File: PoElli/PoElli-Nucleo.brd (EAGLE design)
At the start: 79.5 x 70 mm, 122 parts, among them CN10 NUCLEO-CN10, CN7 NUCLEO-CN7, J3 M022.54MM, J4 M022.54MM, Q3 FDMC2674, Q4 IRFL4310, SW1 A6H2101, SW2 A6H2101, T1 Coilcraft 230NL, T2 FLYBACK750311689, U4 LT3748, U5 TPS2378, U6 ENC424J600, X1 POE-TP-SHIELDED-RJ45-MOLEX-85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, Y1 25 MHz

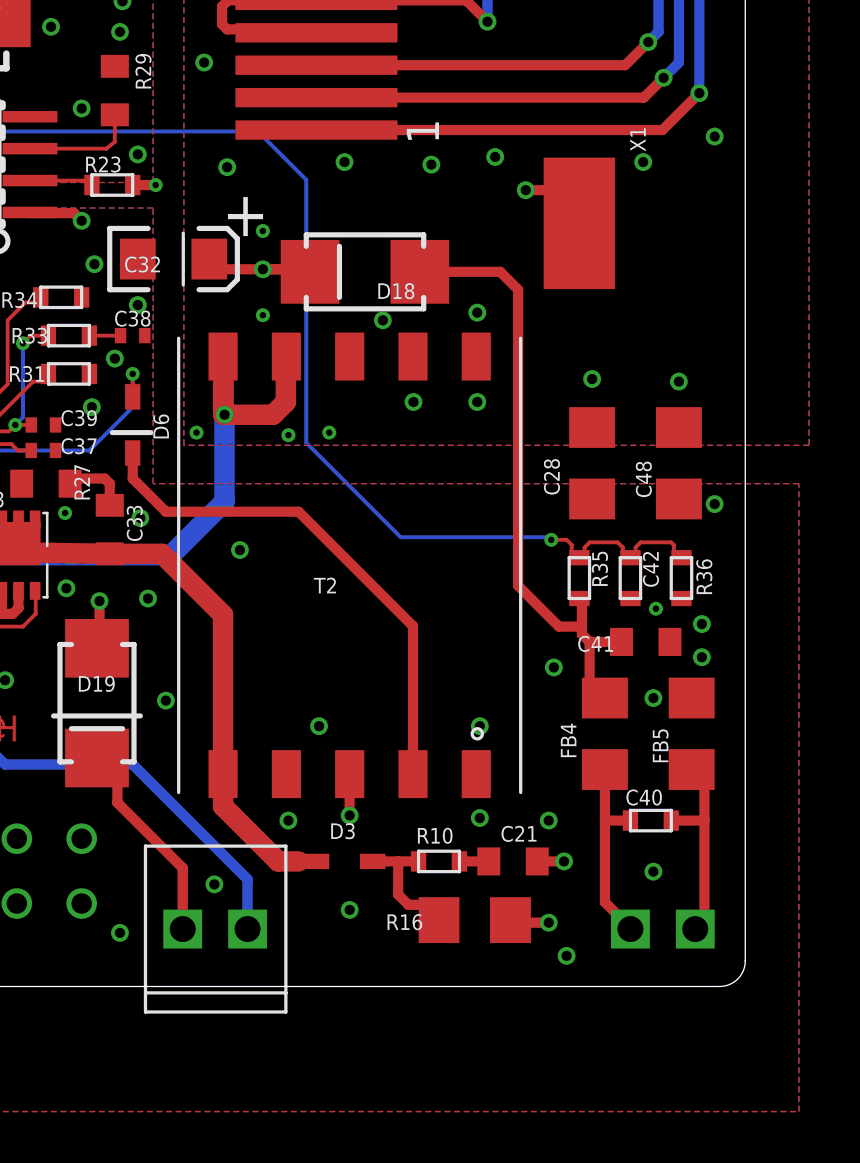
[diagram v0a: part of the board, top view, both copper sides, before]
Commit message: final tweakings, draft v0.9
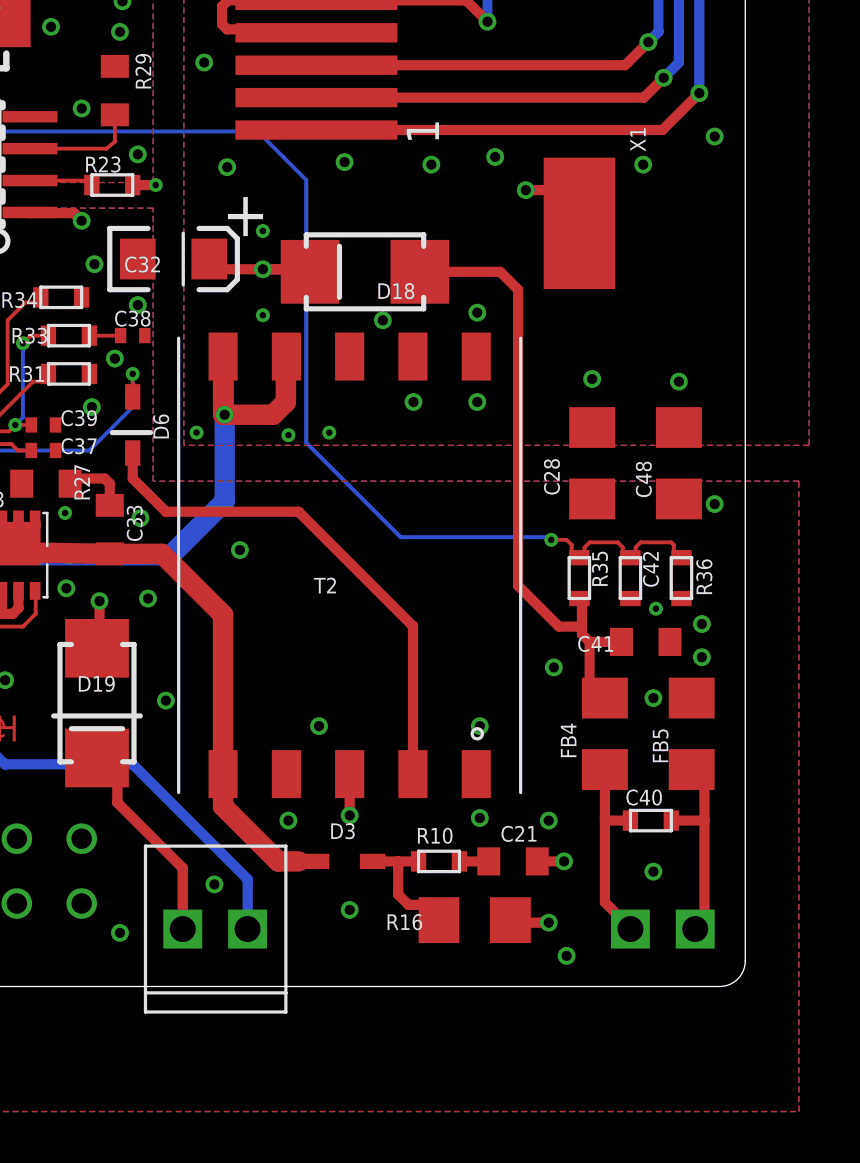
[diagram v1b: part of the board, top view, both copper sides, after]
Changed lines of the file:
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@@
 <layer number="110" name="fp0" color="7" fill="1" visible="no" active="yes"/>
 <layer number="111" name="111" color="7" fill="1" visible="no" active="yes"/>
-<layer number="112" name="tSilk" color="7" fill="1" visible="no" active="yes"/>
-<layer number="113" name="bSilk" color="7" fill="1" visible="no" active="yes"/>
+<layer number="112" name="tSilk" color="7" fill="1" visible="yes" active="yes"/>
+<layer number="113" name="bSilk" color="7" fill="1" visible="yes" active="yes"/>
 <layer number="116" name="Patch_BOT" color="9" fill="4" visible="no" active="yes"/>
 <layer number="118" name="Rect_Pads" color="7" fill="1" visible="no" active="yes"/>
@@
 <contactref element="C48" pad="1"/>
 <polygon width="0.15" layer="16">
-<vertex x="81.6" y="19.7"/>
-<vertex x="56.3" y="19.7"/>
+<vertex x="81.6" y="19.8"/>
+<vertex x="56.3" y="19.8"/>
 <vertex x="56.3" y="30.5"/>
 <vertex x="38" y="30.5"/>
@@
 <via x="78.3" y="18.9" extent="1-16" drill="0.4"/>
 <polygon width="0.15" layer="1">
-<vertex x="81.6" y="19.7"/>
-<vertex x="56.3" y="19.7"/>
+<vertex x="81.6" y="19.8"/>
+<vertex x="56.3" y="19.8"/>
 <vertex x="56.3" y="30.5"/>
 <vertex x="38" y="30.5"/>
@@
 <via x="55.8" y="18.35" extent="1-16" drill="0.4"/>
 <polygon width="0.15" layer="2">
-<vertex x="81.6" y="19.7"/>
-<vertex x="56.3" y="19.7"/>
+<vertex x="81.6" y="19.8"/>
+<vertex x="56.3" y="19.8"/>
 <vertex x="56.3" y="30.5"/>
 <vertex x="38" y="30.5"/>
@@
 <via x="69" y="22.9" extent="1-16" drill="0.4"/>
 <via x="78.3" y="33.3" extent="1-16" drill="0.4"/>
-<via x="75.5" y="32.3" extent="1-16" drill="0.4"/>
+<via x="75.5" y="32.2" extent="1-16" drill="0.4"/>
 <via x="69.7" y="32.5" extent="1-16" drill="0.4"/>
 <via x="63.8" y="32.3" extent="1-16" drill="0.4"/>
@@
 <via x="63.1" y="44.9" extent="1-16" drill="0.4"/>
 <wire x1="63.1" y1="44.9" x2="70.9" y2="44.9" width="0.4" layer="2"/>
-<wire x1="70.9" y1="44.9" x2="73" y2="47" width="0.4" layer="2"/>
-<wire x1="73" y1="47" x2="73" y2="49.2" width="0.4" layer="2"/>
-<wire x1="73" y1="49.2" x2="73.1" y2="49.3" width="0.4" layer="2"/>
+<wire x1="70.9" y1="44.9" x2="73.1" y2="47.1" width="0.4" layer="2"/>
+<wire x1="73.1" y1="47.1" x2="73.1" y2="49.3" width="0.4" layer="2"/>
 <via x="73.1" y="49.3" extent="1-16" drill="0.4"/>
 <wire x1="73.1" y1="49.3" x2="73.1" y2="46.2" width="0.4" layer="1"/>
@@
 <contactref element="D19" pad="A"/>
 <polygon width="0.15" layer="15">
-<vertex x="39.8" y="-2"/>
-<vertex x="39.8" y="22.3"/>
-<vertex x="37.5" y="22.3"/>
-<vertex x="37.5" y="44.8"/>
+<vertex x="37.7" y="-1.9"/>
+<vertex x="37.7" y="44.8"/>
 <vertex x="84" y="44.8"/>
 <vertex x="84" y="-2"/>
@@
 <vertex x="28.2" y="-2.2"/>
 <vertex x="28.2" y="8.4"/>
-<vertex x="18.8" y="8.4"/>
-<vertex x="18.8" y="22.3"/>
-<vertex x="36.4" y="22.3"/>
-<vertex x="36.4" y="46"/>
+<vertex x="19.3" y="8.4"/>
+<vertex x="19.3" y="22.3"/>
+<vertex x="36.9" y="22.3"/>
+<vertex x="36.9" y="46"/>
 <vertex x="81.1" y="46"/>
 <vertex x="81.1" y="70.9"/>
 <vertex x="-2.3" y="70.9"/>
 <vertex x="-2.3" y="48.6"/>
-<vertex x="30.1" y="48.6"/>
-<vertex x="30.1" y="30.6"/>
-<vertex x="9.8" y="30.6"/>
-<vertex x="9.8" y="48.45"/>
-<vertex x="-2.3" y="48.45"/>
+<vertex x="29.9" y="48.6"/>
+<vertex x="29.9" y="30.6"/>
+<vertex x="10" y="30.6"/>
+<vertex x="10" y="48.5"/>
+<vertex x="-2.3" y="48.5"/>
 <vertex x="-2.3" y="-2.2"/>
 </polygon>
@@
 <contactref element="CN7" pad="24"/>
 <polygon width="0.15" layer="15">
-<vertex x="38.8" y="-2"/>
+<vertex x="36.9" y="-2"/>
 <vertex x="29.2" y="-2"/>
 <vertex x="29.2" y="9.4"/>
-<vertex x="19.7" y="9.4"/>
-<vertex x="19.7" y="21.3"/>
-<vertex x="38.8" y="21.3"/>
+<vertex x="20.1" y="9.4"/>
+<vertex x="20.1" y="21.5"/>
+<vertex x="36.9" y="21.5"/>
 </polygon>
 <via x="33.3" y="13.8" extent="1-16" drill="0.4"/>
